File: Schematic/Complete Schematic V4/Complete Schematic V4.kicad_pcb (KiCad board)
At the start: 2 copper layers, 73 parts, among them J1 Conn_Coaxial, J2 USB_A, J3 AudioJack3, U1 Si5351A-B-GT, U2 SN74CBT3253, U3 LT6231, U4 LT6231, U5 LM4562MA, U6 LM4562MA, Y1 Crystal_GND24_Small

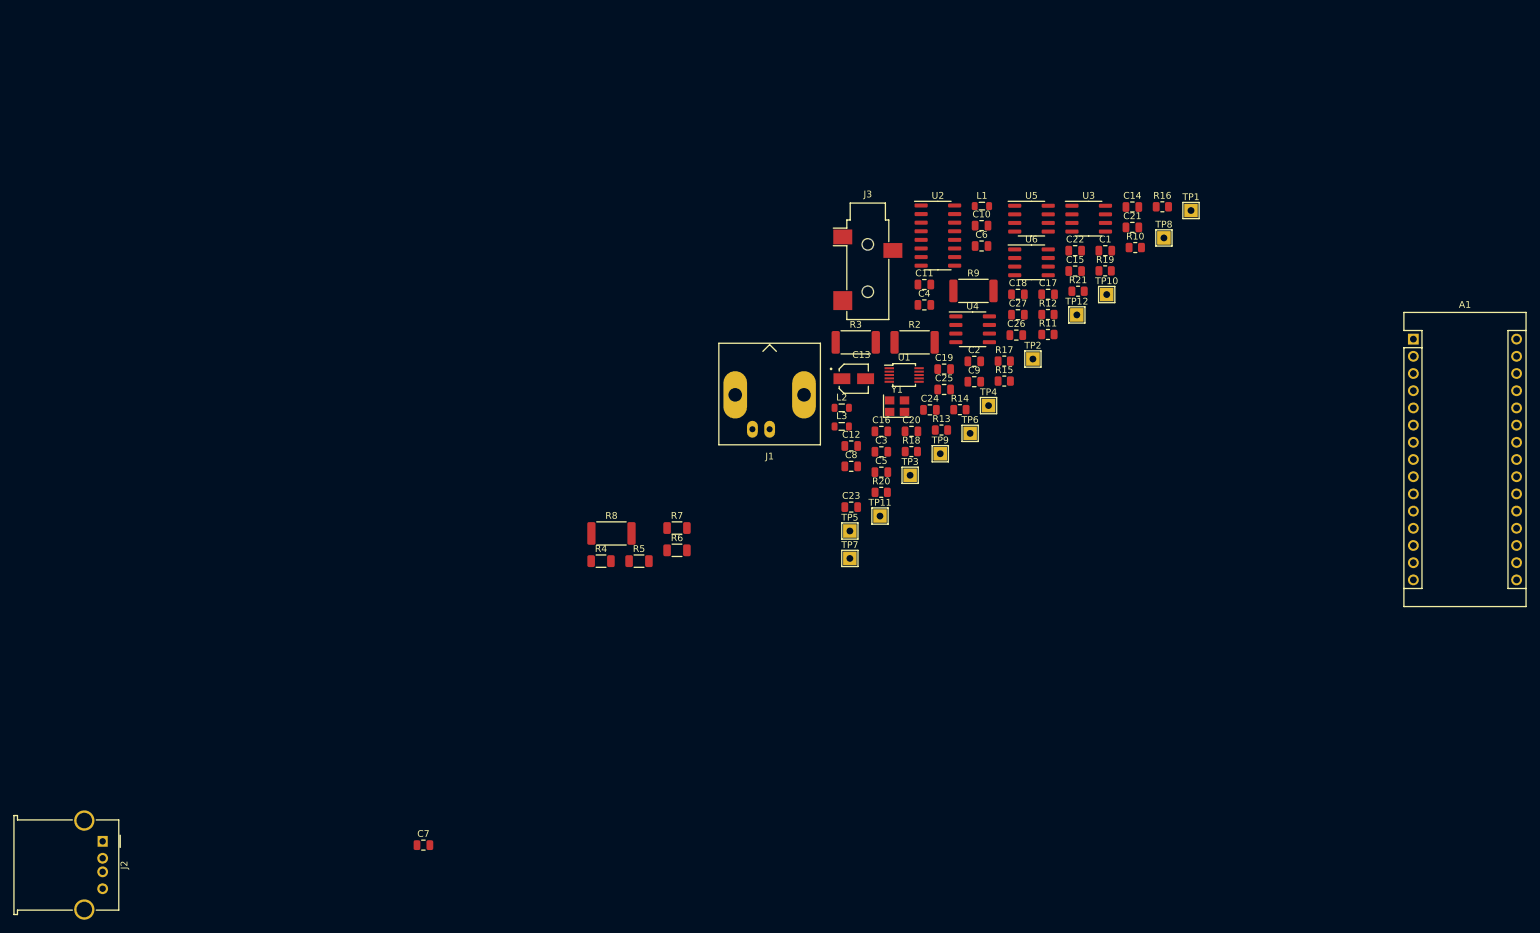
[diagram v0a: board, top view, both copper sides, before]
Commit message: PCB Design
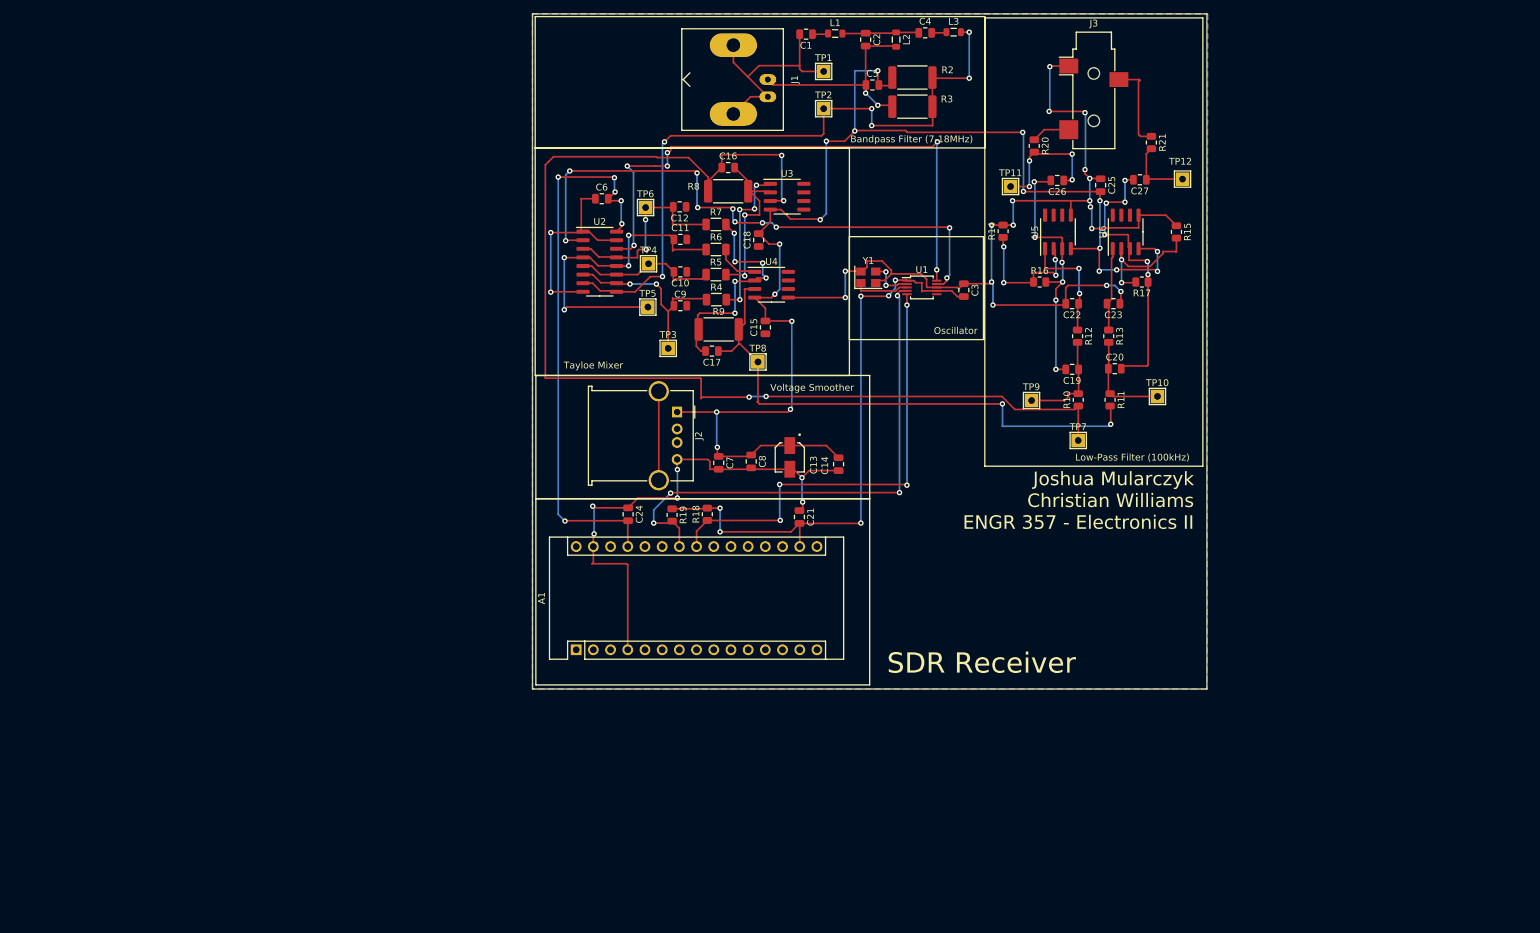
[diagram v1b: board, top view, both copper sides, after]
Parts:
- moved A1 131.9 mm to (107.7, 150.0), turned to 90 degrees
- moved J2 105.9 mm to (122.6, 114.9)
- moved R19 73.4 mm to (121.8, 130.1), turned to -90 degrees
- moved C7 71.3 mm to (128.7, 122.4), turned to -90 degrees
- moved C21 65.2 mm to (140.6, 130.4), turned to -90 degrees
- moved TP8 62.7 mm to (134.5, 107.5)
- moved L3 60.5 mm to (163.4, 58.8)
- moved TP6 58.4 mm to (117.9, 84.7)
- moved TP1 58.0 mm to (144.2, 64.6)
- moved C14 57.7 mm to (146.4, 122.6), turned to 90 degrees
- moved C5 57.2 mm to (151.4, 66.6)
- moved C6 56.5 mm to (111.4, 83.4)
- moved R20 55.9 mm to (175.3, 75.6), turned to -90 degrees
- moved L2 55.0 mm to (154.9, 59.9), turned to -90 degrees
- moved C1 54.5 mm to (141.6, 59.1), turned to 180 degrees
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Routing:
- net GND: track 0.00 -> 284.7 mm, vias 0 -> 27
- net Filtered 5V: track 0.00 -> 201.7 mm, vias 0 -> 18
- net Net-(C16-Pad1): track 0.00 -> 171.2 mm, vias 0 -> 4
- net Net-(L3-Pad2): track 0.00 -> 100.1 mm, vias 0 -> 6
- net +3V3: track 0.00 -> 87.7 mm, vias 0 -> 6
- net Net-(U1-Pad9): track 0.00 -> 86.3 mm, vias 0 -> 10
- net Net-(U1-Pad10): track 0.00 -> 84.2 mm, vias 0 -> 6
- net +5V: track 0.00 -> 83.3 mm, vias 0 -> 6
- net Net-(C17-Pad1): track 0.00 -> 81.8 mm, vias 0 -> 2
- net /SCL: track 0.00 -> 77.4 mm, vias 0 -> 4
- net /SDA: track 0.00 -> 67.7 mm, vias 0 -> 4
- net Net-(C11-Pad1): track 0.00 -> 48.5 mm, vias 0 -> 4
- net Net-(C20-Pad2): track 0.00 -> 42.9 mm, vias 0 -> 6
- net Net-(C19-Pad2): track 0.00 -> 38.6 mm, vias 0 -> 6
- net Net-(C17-Pad2): track 0.00 -> 34.2 mm, vias 0 -> 6
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- added copper zone on B.Cu, net GND
- added copper zone on F.Cu, net GND
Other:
- board outline added: 99.6 x 99.7 mm
- board text added: "Bandpass Filter (7-18MHz)"
- board text added: "Joshua Mularczyk Christian Williams ENGR 357 - Electronics II"
- board text added: "Low-Pass Filter (100kHz)"
- board text added: "Oscillator"
- board text added: "SDR Receiver"
- board text added: "Tayloe Mixer"
- board text added: "Voltage Smoother"
